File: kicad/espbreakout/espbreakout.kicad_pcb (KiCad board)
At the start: 2 copper layers, 48.3 x 71.1 mm, 27 parts, among them J1 TEMPERATURE, J2 POWER, J3 CURRENT, J4 LED DATA, J5 RELAY, J6 Conn_01x19, J7 Conn_01x19, J8 I2C, J9 SERIAL

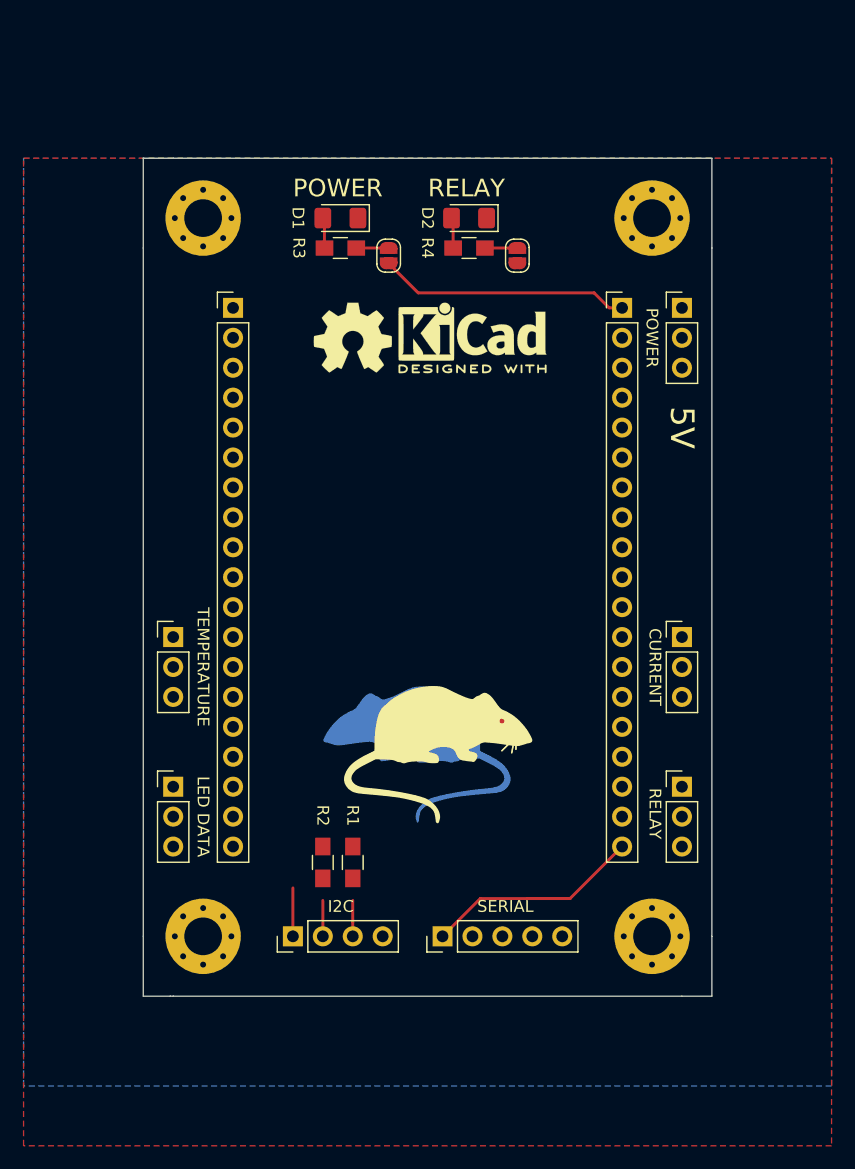
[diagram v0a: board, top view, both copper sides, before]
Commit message: esp breakout
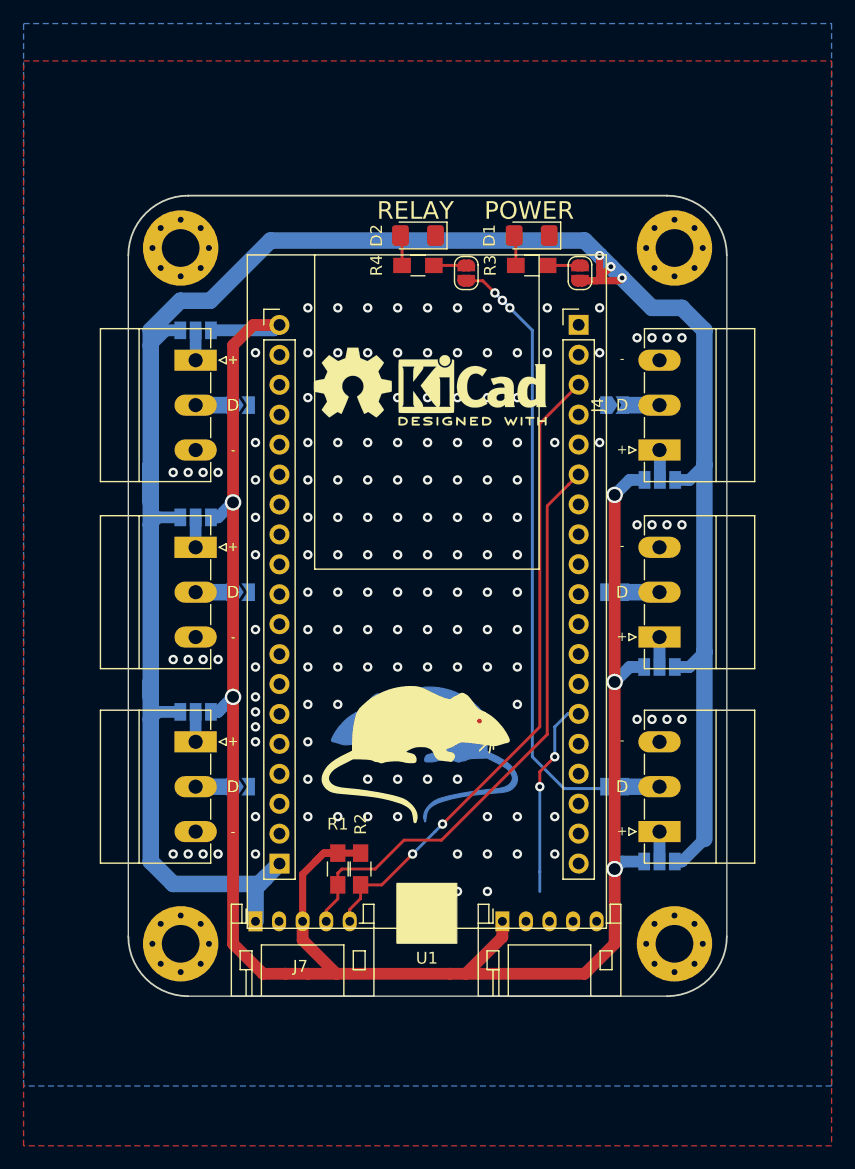
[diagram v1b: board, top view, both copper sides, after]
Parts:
- removed the J6 at (38.1, 20.3)
- removed the J8 at (43.2, 73.7)
- added J3: UNK, Connectors_Phoenix:PhoenixContact_MC-G_03x3.81mm_Angled, F.Cu at (34.9, 24.8)
- added JP10: Jumper_3_Open, Jumper:SolderJumper-3_P1.3mm_Open_Pad1.0x1.5mm, B.Cu at (74.3, 50.8)
- added JP11: Jumper_3_Open, Jumper:SolderJumper-3_P1.3mm_Open_Pad1.0x1.5mm, B.Cu at (34.9, 54.6)
- added JP12: Jumper_3_Open, Jumper:SolderJumper-3_P1.3mm_Open_Pad1.0x1.5mm, B.Cu at (74.3, 67.3)
- added JP13: Jumper_3_Open, Jumper:SolderJumper-3_P1.3mm_Open_Pad1.0x1.5mm, B.Cu at (34.9, 22.2)
- added JP14: SolderJumper_2_Open, Jumper:SolderJumper-2_P1.3mm_Open_TrianglePad1.0x1.5mm, B.Cu at (38.7, 28.6)
- added JP3: SolderJumper_2_Open, Jumper:SolderJumper-2_P1.3mm_Open_TrianglePad1.0x1.5mm, B.Cu at (38.7, 44.5)
- added JP4: D, Jumper:SolderJumper-2_P1.3mm_Open_TrianglePad1.0x1.5mm, B.Cu at (70.5, 28.6)
- added JP5: SolderJumper_2_Open, Jumper:SolderJumper-2_P1.3mm_Open_TrianglePad1.0x1.5mm, B.Cu at (38.7, 61.0)
- added JP6: D, Jumper:SolderJumper-2_P1.3mm_Open_TrianglePad1.0x1.5mm, B.Cu at (70.5, 44.5)
- added JP7: D, Jumper:SolderJumper-2_P1.3mm_Open_TrianglePad1.0x1.5mm, B.Cu at (70.5, 61.0)
- added JP8: Jumper_3_Open, Jumper:SolderJumper-3_P1.3mm_Open_Pad1.0x1.5mm, B.Cu at (34.9, 38.1)
- added JP9: Jumper_3_Open, Jumper:SolderJumper-3_P1.3mm_Open_Pad1.0x1.5mm, B.Cu at (74.3, 34.9)
- added U1: ESP32-38pins, drz-lib:esp32 38pin azdelivery, F.Cu at (54.5, 44.4)
- J1: footprint Pin_Headers:Pin_Header_Straight_1x03_Pitch2.54mm -> Connectors_Phoenix:PhoenixContact_MC-G_03x3.81mm_Angled
- J2: renamed from J4; footprint Pin_Headers:Pin_Header_Straight_1x03_Pitch2.54mm -> Connectors_Phoenix:PhoenixContact_MC-G_03x3.81mm_Angled
- J4: renamed from J2; footprint Pin_Headers:Pin_Header_Straight_1x03_Pitch2.54mm -> Connectors_Phoenix:PhoenixContact_MC-G_03x3.81mm_Angled
- J5: renamed from J3; footprint Pin_Headers:Pin_Header_Straight_1x03_Pitch2.54mm -> Connectors_Phoenix:PhoenixContact_MC-G_03x3.81mm_Angled
- J6: renamed from J5; footprint Pin_Headers:Pin_Header_Straight_1x03_Pitch2.54mm -> Connectors_Phoenix:PhoenixContact_MC-G_03x3.81mm_Angled
- J7: value Conn_01x19 -> I2C; footprint Pin_Headers:Pin_Header_Straight_1x19_Pitch2.54mm -> Connectors_JST:JST_PH_S5B-PH-K_05x2.00mm_Angled
- J8: renamed from J9; footprint Pin_Headers:Pin_Header_Straight_1x05_Pitch2.54mm -> Connectors_JST:JST_PH_S5B-PH-K_05x2.00mm_Angled
- moved J7 60.7 mm to (40.0, 72.4)
- moved JP1 16.3 mm to (67.5, 17.4)
- moved D1 16.3 mm to (63.4, 14.2)
- moved R3 16.3 mm to (63.4, 16.7)
- moved J4 12.2 mm to (74.3, 32.4), turned to 90 degrees
- moved J1 7.85 mm to (34.9, 40.6), turned to 270 degrees
- moved J8 5.24 mm to (61.0, 72.4), turned to 0 degrees
- moved D2 4.58 mm to (53.8, 14.2)
- moved R4 4.58 mm to (53.8, 16.7)
- moved JP2 4.58 mm to (57.9, 17.4)
- moved REF*** 4.45 mm to (58.4, 27.3)
- moved REF*** 4.45 mm to (61.0, 27.3)
- moved REF*** 4.45 mm to (50.8, 27.3)
- moved J2 4.26 mm to (34.9, 57.1), turned to 270 degrees
- moved J6 4.26 mm to (74.3, 64.8), turned to 90 degrees
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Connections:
- J1 pad 1: (no net) -> Net-(J1-Pad1)
- J1 pad 2: (no net) -> Net-(J1-Pad2)
- J2 pad 1: (no net) -> Net-(J2-Pad1)
- J2 pad 2: (no net) -> Net-(J2-Pad2)
- J4 pad 1: 5V -> Net-(J4-Pad1)
- J4 pad 2: (no net) -> Net-(J4-Pad2)
- J5 pad 1: (no net) -> Net-(J5-Pad1)
- J5 pad 2: (no net) -> Net-(J5-Pad2)
- J6 pad 1: (no net) -> Net-(J6-Pad1)
- J6 pad 2: RELAY_TRIGGER -> Net-(J6-Pad2)
- J7 pad 2: (no net) -> GND
- J7 pad 3: (no net) -> 3V3
- J7 pad 4: (no net) -> SDA
- J7 pad 5: (no net) -> SCL
- J8 pad 2: (no net) -> TX
- J8 pad 3: (no net) -> RX
- J8 pad 4: (no net) -> GPIO0
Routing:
- net 5V: track 21.4 -> 189.3 mm, vias 0 -> 3
- net 3V3: track 25.9 -> 171.6 mm, vias 0 -> 5
- net RELAY_TRIGGER: track 0.00 -> 52.8 mm, vias 0 -> 3
- net SCL: track 3.05 -> 55.3 mm, vias 0 -> 2
- net SDA: track 3.05 -> 50.3 mm
- net GPIO0: track 0.00 -> 17.0 mm, vias 0 -> 2
- net Net-(J3-Pad2): track 0.00 -> 3.09 mm
- net Net-(J2-Pad2): track 0.00 -> 3.09 mm
- net Net-(J1-Pad2): track 0.00 -> 3.09 mm
- net Net-(J6-Pad2): track 0.00 -> 2.63 mm
- net Net-(J5-Pad2): track 0.00 -> 2.63 mm
- net Net-(J4-Pad1): track 0.00 -> 2.55 mm
- net Net-(J6-Pad1): track 0.00 -> 2.54 mm
- net Net-(J4-Pad2): track 0.00 -> 2.54 mm
- net Net-(J5-Pad1): track 0.00 -> 2.54 mm
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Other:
- board size 48.3 x 71.1 mm -> 50.8 x 67.9 mm
- board text added: "+"
- board text added: "-"
- board text added: "3V"
- board text added: "3V3"
- board text added: "BTL"
- board text added: "D"
- board text added: "GND"
- board text added: "RX"
- board text added: "SCL"
- board text added: "SDA"
- board text added: "TX"
